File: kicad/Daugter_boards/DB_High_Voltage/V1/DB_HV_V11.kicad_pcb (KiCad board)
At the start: 2 copper layers, 57.2 x 50.8 mm, 38 parts, among them P1 CONN_01X19, P2 CONN_01X02, P3 CONN_01X19, P4 SMA, Q1 QN2222, Q2 QN2222, Q3 Q2N2907, U1 LM555N

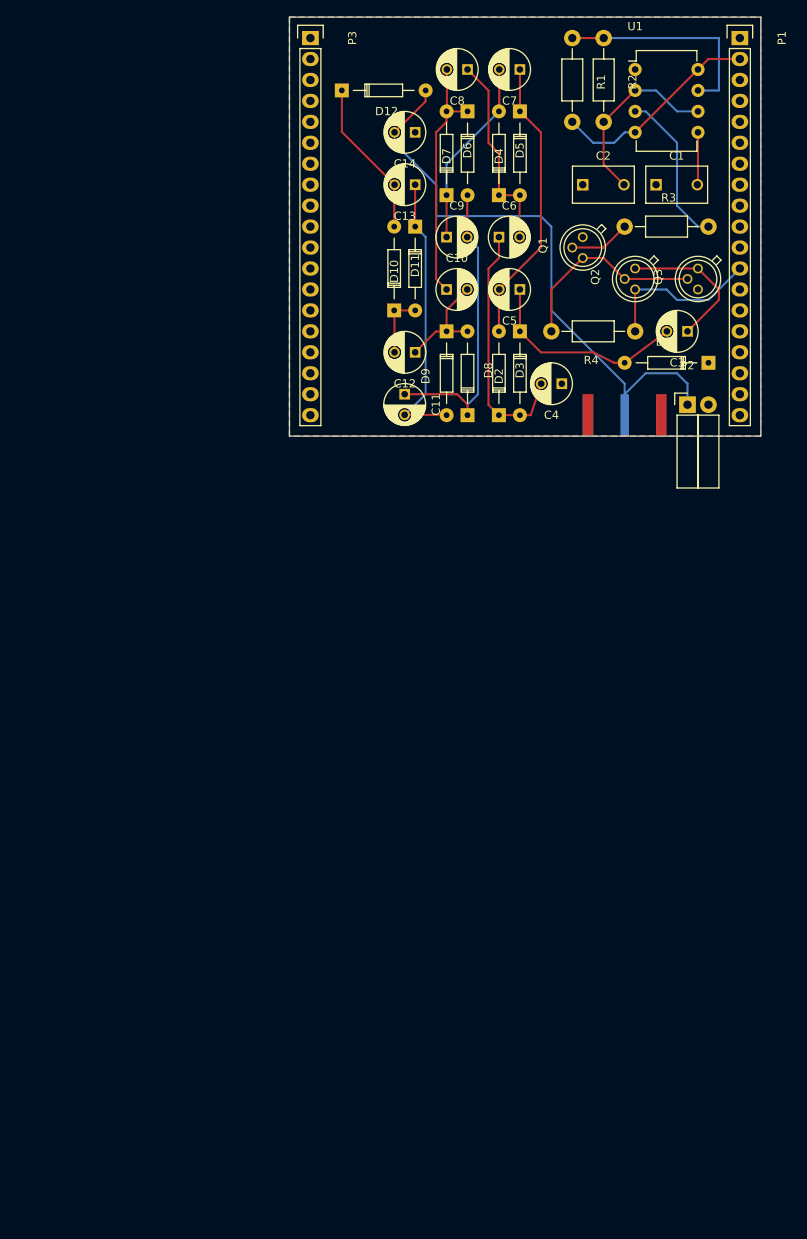
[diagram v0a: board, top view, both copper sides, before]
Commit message: update DB_HV_V1
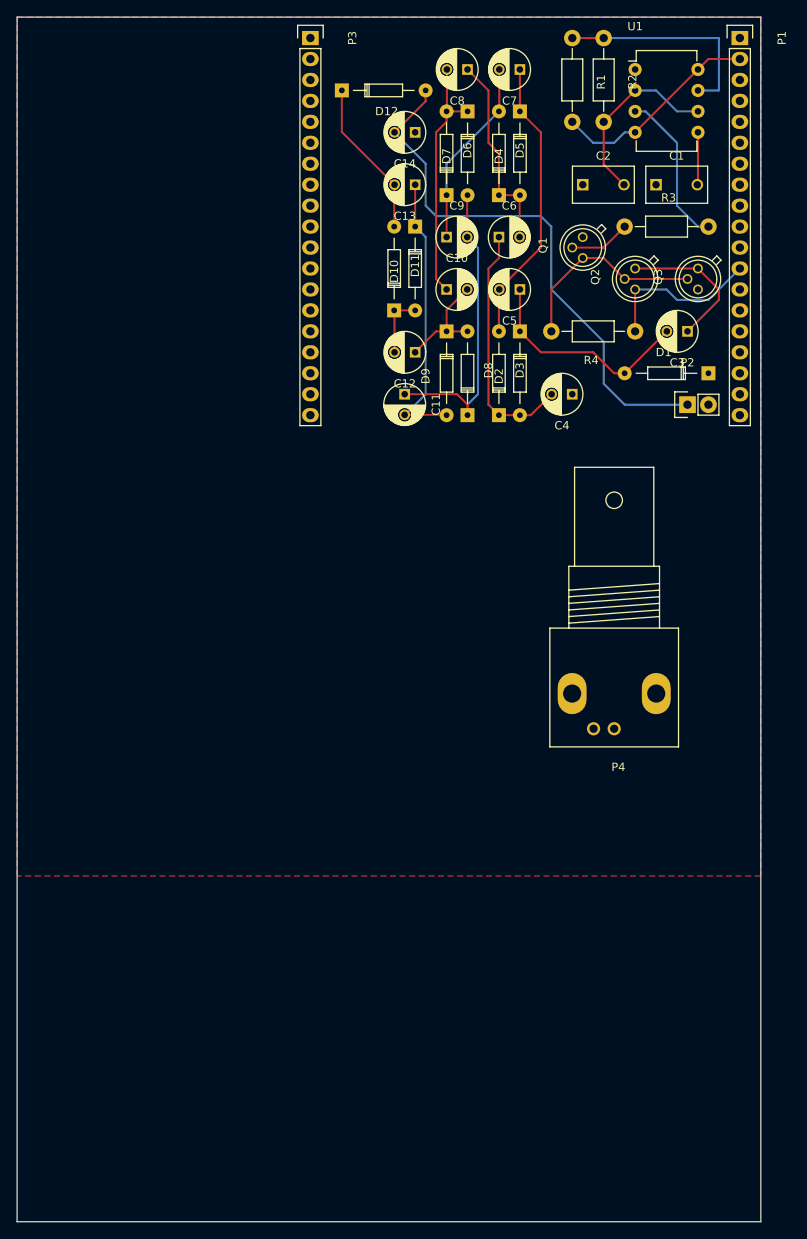
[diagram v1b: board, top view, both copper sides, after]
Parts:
- P2: footprint Socket_Strips:Socket_Strip_Angled_1x02 -> Socket_Strips:Socket_Strip_Straight_1x02
- P4: footprint echopen:SMA -> Sockets_BNC:BNC_Socket_TYCO-AMP; moved to F.Cu
- moved P4 33.0 mm to (110.5, 114.3)
- moved C4 1.80 mm to (105.4, 78.7)
- moved D1 1.27 mm to (121.9, 76.2)
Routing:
- net Net-(C14-Pad2): track 74.2 -> 66.3 mm
- net Net-(C3-Pad2): track 25.5 -> 27.1 mm
- removed copper zone on B.Cu, net GND
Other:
- board size 57.2 x 50.8 mm -> 90.2 x 146 mm
